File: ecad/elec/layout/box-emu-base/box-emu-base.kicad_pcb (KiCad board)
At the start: 2 copper layers, 72.5 x 63.9 mm, 69 parts

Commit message: minor update
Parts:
- MECH1, MECH2: value (none) -> SILKSCREENGBC_A/B
- REF**: value (none) -> BOX_EMU_BASE
- U$1: value (none) -> SILKSCREENGBC_D-PAD
- U$2: value (none) -> SILKSCREENGBC_START/SELECT

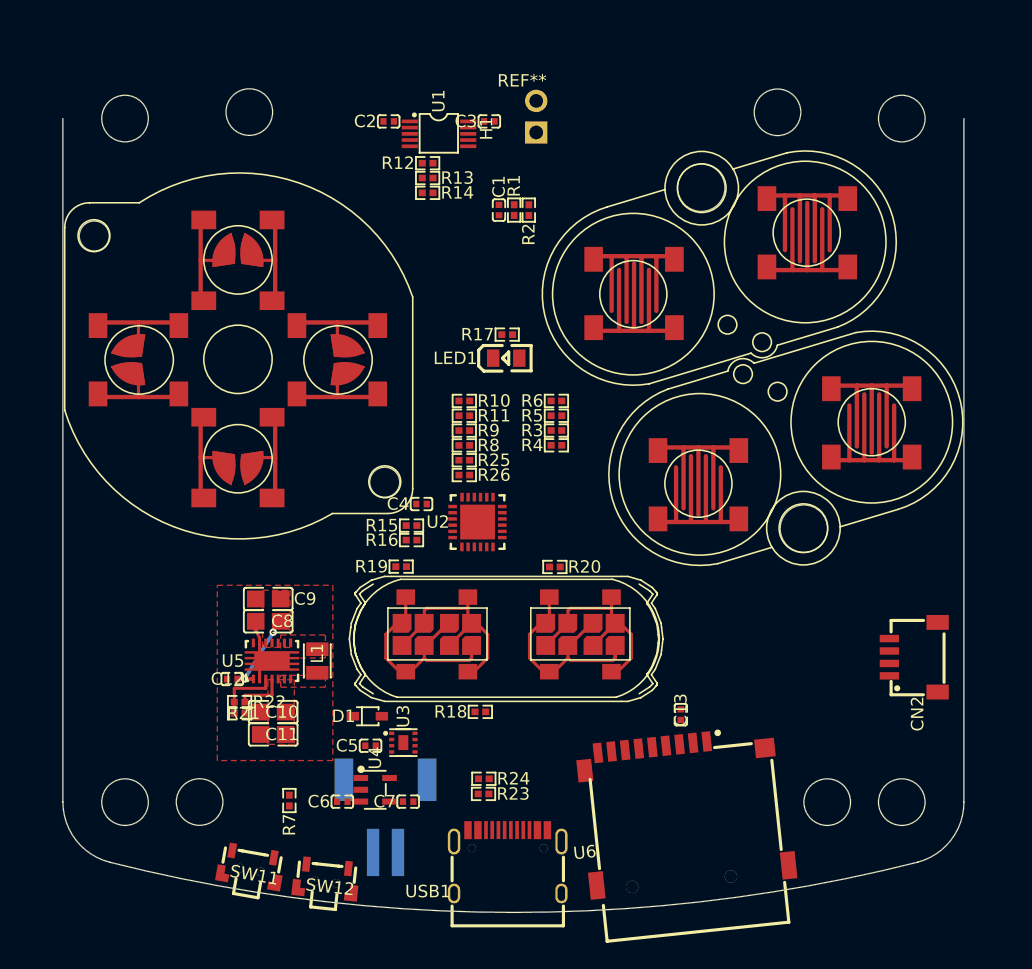
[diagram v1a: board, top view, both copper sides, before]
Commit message: simple layout
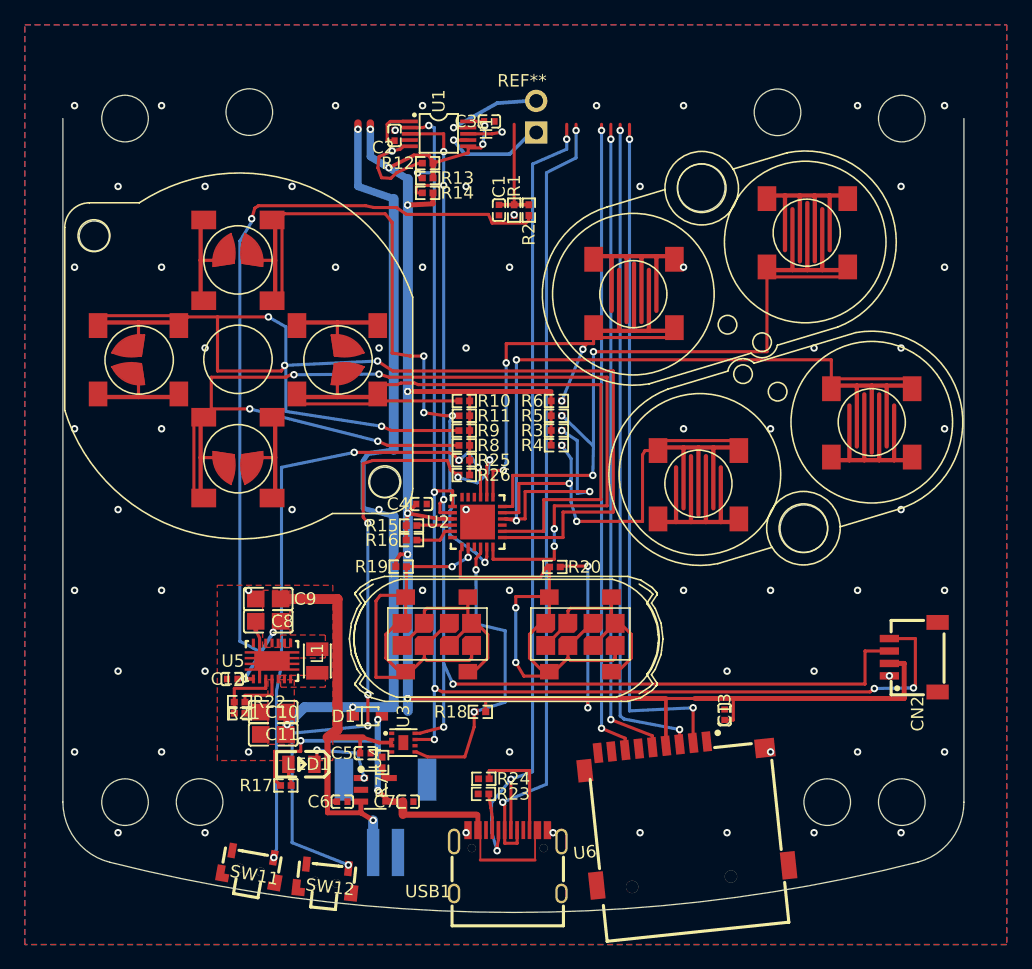
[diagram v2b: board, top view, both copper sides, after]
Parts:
- moved R17 40.4 mm to (117.4, 128.6)
- moved LED1 36.6 mm to (118.7, 126.9), turned to 180 degrees
- moved R7 8.07 mm to (125.2, 126.8)
- moved C13 3.52 mm to (152.7, 122.9)
- moved C2 1.23 mm to (126.2, 76.3), turned to 90 degrees
- moved C5 0.73 mm to (123.8, 126.0)
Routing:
- net vcc_3v3: track 0.00 -> 161.2 mm, vias 0 -> 11
- net SCL: track 0.00 -> 101.6 mm, vias 0 -> 7
- net vbat: track 5.69 -> 102.6 mm, vias 2 -> 4
- net SDA: track 0.00 -> 96.3 mm, vias 0 -> 5
- net left: track 0.00 -> 96.2 mm, vias 0 -> 4
- net down: track 0.00 -> 87.6 mm, vias 0 -> 6
- net DATA_N: track 0.00 -> 67.4 mm, vias 0 -> 3
- net line: track 0.00 -> 64.9 mm, vias 0 -> 4
- net DATA_P: track 0.00 -> 63.8 mm, vias 0 -> 2
- net vcc_5v: track 4.04 -> 67.6 mm, vias 0 -> 4
- net vol_up: track 0.00 -> 56.1 mm, vias 0 -> 6
- net cs-2: track 0.00 -> 55.2 mm, vias 0 -> 2
- net MOSI: track 0.00 -> 53.7 mm, vias 0 -> 2
- net SCLK: track 0.00 -> 52.4 mm, vias 0 -> 2
- net up: track 0.00 -> 52.3 mm, vias 0 -> 4
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- added copper zone on B.Cu, net gnd
